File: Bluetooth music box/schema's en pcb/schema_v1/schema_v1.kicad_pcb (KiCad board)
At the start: 4 copper layers, 141 x 87.6 mm, 151 parts, among them J1 Pickit aansluiting, J2 USB_B_Micro, SW1 SW_Push, SW3 SW_Push, SW4 SW_Push, SW5 SW_Push, SW6 SW_Push, SW7 SW_Push, SW9 Switch, U1 LTC2063, U10 SN74LVC1T45DBV, U11 tpa3140, U12 LTC4001, U14 TPS563200, U2 pic18f27k40, U5 FT232RL, U6 LM1117-3.3, U8 OVC3860_EDR, U9 Spi_header

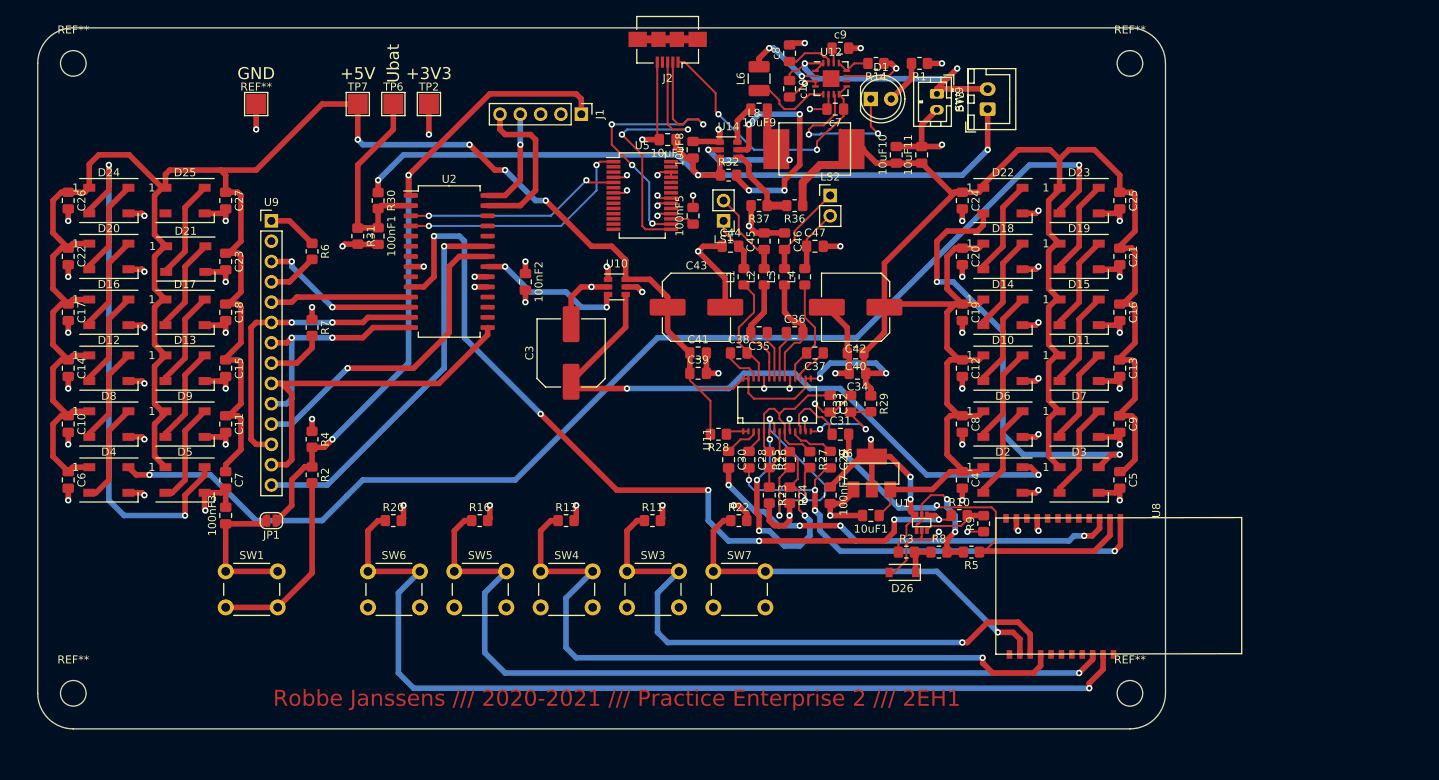
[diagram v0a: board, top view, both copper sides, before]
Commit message: Nieuwe start
Nieuw schema (andere µC, BT-module, dc/dc, verschillversterkers)
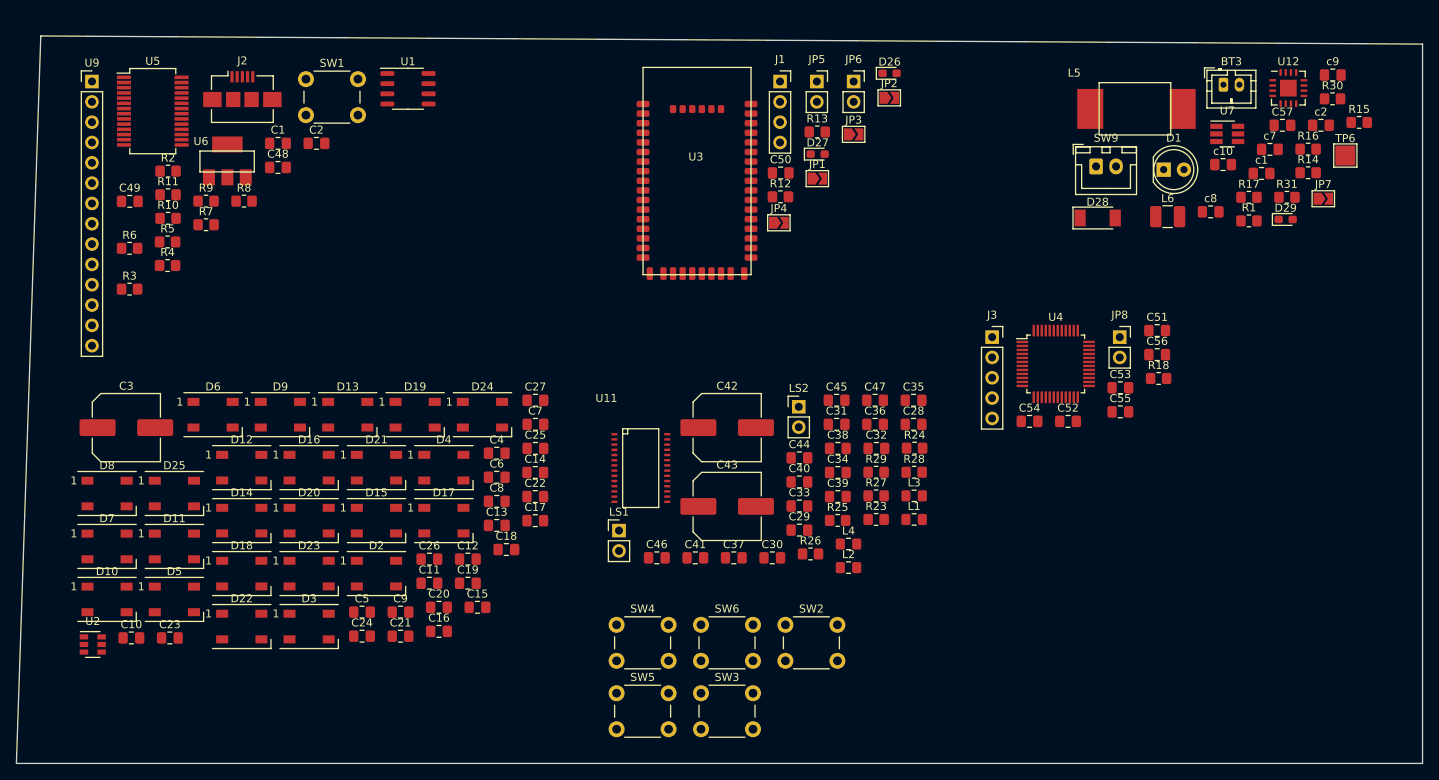
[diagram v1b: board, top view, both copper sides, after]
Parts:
- removed 100nF1, 100nF2, 100nF3, 100nF5, 100nF7, 10uF1, 10uF7, 10uF8: C, Capacitor_SMD:C_0805_2012Metric_Pad1.18x1.45mm_HandSolder
- removed 10uF10, 10uF11: 22µF, Capacitor_SMD:C_0805_2012Metric_Pad1.18x1.45mm_HandSolder
- removed 10uF9: 0.1µF, Capacitor_SMD:C_0805_2012Metric_Pad1.18x1.45mm_HandSolder
- removed L8: 2.2uH, Robbe_modules:L_tps563200
- removed R20, R22, R32, R37: 10k, Resistor_SMD:R_0805_2012Metric_Pad1.20x1.40mm_HandSolder
- removed R36: 56k, Resistor_SMD:R_0805_2012Metric_Pad1.20x1.40mm_HandSolder
- removed REF**: TestPoint_GND, TestPoint:TestPoint_Pad_2.5x2.5mm
- removed REF** (x4): MountingHole_3.2mm_M3, MountingHole:MountingHole_3.2mm_M3
- removed SW7: SW_Push, Button_Switch_THT:SW_PUSH_6mm_H7.3mm
- removed TP2, TP7: TestPoint, TestPoint:TestPoint_Pad_2.5x2.5mm
- removed U10: SN74LVC1T45DBV, Package_TO_SOT_SMD:SOT-23-6
- removed U14: TPS563200, Package_TO_SOT_SMD:SOT-23-6
- removed U8: OVC3860_EDR, Robbe_modules:OVC3860_EDR
- added C1: 100nF, Capacitor_SMD:C_0805_2012Metric_Pad1.18x1.45mm_HandSolder, F.Cu at (106.9, 62.7)
- added C2: 10uF, Capacitor_SMD:C_0805_2012Metric_Pad1.18x1.45mm_HandSolder, F.Cu at (111.7, 62.7)
- added C48: 100nF, Capacitor_SMD:C_0805_2012Metric_Pad1.18x1.45mm_HandSolder, F.Cu at (106.9, 65.7)
- added C49: 100nF, Capacitor_SMD:C_0805_2012Metric_Pad1.18x1.45mm_HandSolder, F.Cu at (88.3, 70.0)
- added C50: 10uF, Capacitor_SMD:C_0805_2012Metric_Pad1.18x1.45mm_HandSolder, F.Cu at (169.7, 66.4)
- added C51: 100nF, Capacitor_SMD:C_0805_2012Metric_Pad1.18x1.45mm_HandSolder, F.Cu at (216.8, 86.1)
- added C52: 100nF, Capacitor_SMD:C_0805_2012Metric_Pad1.18x1.45mm_HandSolder, F.Cu at (205.6, 97.5)
- added C53: 100nF, Capacitor_SMD:C_0805_2012Metric_Pad1.18x1.45mm_HandSolder, F.Cu at (212.2, 93.3)
- added C54: 100nF, Capacitor_SMD:C_0805_2012Metric_Pad1.18x1.45mm_HandSolder, F.Cu at (200.8, 97.5)
- added C55: 100nF, Capacitor_SMD:C_0805_2012Metric_Pad1.18x1.45mm_HandSolder, F.Cu at (212.2, 96.3)
- added C56: 10nF, Capacitor_SMD:C_0805_2012Metric_Pad1.18x1.45mm_HandSolder, F.Cu at (216.8, 89.1)
- added C57: 100nF, Capacitor_SMD:C_0805_2012Metric_Pad1.18x1.45mm_HandSolder, F.Cu at (232.4, 60.4)
- added D27: RED, LED_SMD:LED_0603_1608Metric_Pad1.05x0.95mm_HandSolder, F.Cu at (174.3, 64.0)
- added D28: D_Schottky, Diode_SMD:D_SOD-128, F.Cu at (209.3, 72.0)
- added D29: RED, LED_SMD:LED_0603_1608Metric_Pad1.05x0.95mm_HandSolder, F.Cu at (232.8, 72.2)
- added J3: Conn_01x05_Male, Connector_PinSocket_2.54mm:PinSocket_1x05_P2.54mm_Vertical, F.Cu at (196.1, 86.9)
- added JP2: SolderJumper, Jumper:SolderJumper-2_P1.3mm_Open_TrianglePad1.0x1.5mm, F.Cu at (183.3, 57.0)
- added JP3: SolderJumper, Jumper:SolderJumper-2_P1.3mm_Open_TrianglePad1.0x1.5mm, F.Cu at (178.8, 61.6)
- added JP4: SolderJumper, Jumper:SolderJumper-2_P1.3mm_Open_TrianglePad1.0x1.5mm, F.Cu at (169.5, 72.6)
- added JP5: Jumper, Connector_PinSocket_2.54mm:PinSocket_1x02_P2.54mm_Vertical, F.Cu at (174.2, 55.0)
- added JP6: Jumper, Connector_PinSocket_2.54mm:PinSocket_1x02_P2.54mm_Vertical, F.Cu at (178.8, 55.0)
- added JP7: SolderJumper, Jumper:SolderJumper-2_P1.3mm_Open_TrianglePad1.0x1.5mm, F.Cu at (237.5, 69.6)
- added JP8: Jumper, Connector_PinSocket_2.54mm:PinSocket_1x02_P2.54mm_Vertical, F.Cu at (212.1, 86.9)
- added L5: 2.2uH, Robbe_modules:L_tps563200, F.Cu at (206.4, 53.4)
- added R12: 100, Resistor_SMD:R_0805_2012Metric_Pad1.20x1.40mm_HandSolder, F.Cu at (169.7, 69.4)
- added R15: 562K, Resistor_SMD:R_0805_2012Metric_Pad1.20x1.40mm_HandSolder, F.Cu at (242.0, 60.1)
- added R17: 100, Resistor_SMD:R_0805_2012Metric_Pad1.20x1.40mm_HandSolder, F.Cu at (228.2, 69.4)
- added R18: 10K, Resistor_SMD:R_0805_2012Metric_Pad1.20x1.40mm_HandSolder, F.Cu at (216.9, 92.1)
- added SW2: SW_Push, Button_Switch_THT:SW_PUSH_6mm_H7.3mm, F.Cu at (170.3, 122.9)
- added U3: RN52, Robbe_modules:RN52, F.Cu at (152.5, 79.1)
- added U4: STM32L443CCTx, Package_QFP:LQFP-48_7x7mm_P0.5mm, F.Cu at (204.1, 90.3)
- added U7: TLV61048, Package_TO_SOT_SMD:SOT-23-6_Handsoldering, F.Cu at (225.5, 61.5)
- added c1: 1uF, Capacitor_SMD:C_0805_2012Metric_Pad1.18x1.45mm_HandSolder, F.Cu at (229.8, 66.5)
- added c2: 10µF, Capacitor_SMD:C_0805_2012Metric_Pad1.18x1.45mm_HandSolder, F.Cu at (237.2, 60.4)
- D26: value D_Zener -> BLUE; footprint Diode_SMD:D_SOD-123 -> LED_SMD:LED_0603_1608Metric_Pad1.05x0.95mm_HandSolder
- J1: value Pickit aansluiting -> Conn_01x04; footprint Connector_PinHeader_2.54mm:PinHeader_1x05_P2.54mm_Vertical -> Connector_PinSocket_2.54mm:PinSocket_1x04_P2.54mm_Vertical
- JP1: footprint Jumper:SolderJumper-2_P1.3mm_Open_RoundedPad1.0x1.5mm -> Jumper:SolderJumper-2_P1.3mm_Open_TrianglePad1.0x1.5mm
- R10, R11, R4: value 10k -> 220K
- R13: value 10k -> 100
- R16: value 10k -> 107K
- R2: value 100 -> 100K
- R3: value 10k -> 100K
- R5: value 100k -> 220K
- R8, R9: value 100k -> 100K
- U1: value LTC2063 -> TL072; footprint Robbe_modules:LTC2063 -> Package_SO:SO-8_3.9x4.9mm_P1.27mm
- U2: value pic18f27k40 -> SN74LVC1T45DBV; footprint Package_SO:SOIC-28W_7.5x18.7mm_P1.27mm -> Package_TO_SOT_SMD:SOT-23-6
- moved D7 122.5 mm to (85.5, 113.1)
- moved R30 120.0 mm to (238.7, 57.1), turned to 0 degrees
- moved TP6 119.2 mm to (240.3, 64.2)
- moved R31 116.2 mm to (233.0, 69.4), turned to 0 degrees
- moved D10 115.7 mm to (85.5, 119.7)
- moved D11 115.3 mm to (93.9, 113.1)
- moved R16 113.5 mm to (235.6, 63.4)
- moved D22 109.0 mm to (102.3, 123.1)
- moved R5 107.7 mm to (93.1, 75.0), turned to 0 degrees
- moved D23 107.0 mm to (110.8, 116.5)
- moved R10 105.6 mm to (93.1, 72.1)
- moved R9 105.2 mm to (97.9, 69.9), turned to 0 degrees
- moved D18 103.1 mm to (102.3, 116.5)
- moved R3 102.5 mm to (88.3, 80.9)
- moved C21 101.7 mm to (122.2, 124.3), turned to 0 degrees
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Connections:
- C28 pad 2: /Class d amplifier/Agnd -> /L-
- C29 pad 2: /Class d amplifier/Agnd -> /R-
- C3 pad 1: DataLeds -> +5V
- C30 pad 2: /Class d amplifier/Aleft -> /L+
- C31 pad 2: VoL_Measure -> /R+
- D2 pad 4: DataLeds -> /LEDS/FirstLED
- D26 pad 2: GND -> +3V3
- J1 pad 1: Reset -> Net-(J1-Pad1)
- J1 pad 2: +3V3 -> Net-(J1-Pad2)
- J1 pad 3: GND -> Net-(J1-Pad3)
- J1 pad 4: PGD -> Net-(J1-Pad4)
- JP1 pad 1: Reset -> RTS_BT
- JP1 pad 2: Net-(100nF3-Pad1) -> Net-(J1-Pad1)
- R10 pad 1: Vol_spkr -> GND
- R11 pad 1: vol+ -> /R_SE
- R11 pad 2: GND -> Net-(R11-Pad2)
- R13 pad 1: vol- -> Net-(R13-Pad1)
- R13 pad 2: GND -> Net-(D27-Pad1)
- R16 pad 1: next -> Net-(R15-Pad2)
- R2 pad 1: Reset -> Net-(R2-Pad1)
- R2 pad 2: Net-(R2-Pad2) -> /L+
- R3 pad 1: +3V3 -> Net-(R3-Pad1)
- R3 pad 2: Net-(D26-Pad1) -> /L-
- R4 pad 1: +3V3 -> GND
- R4 pad 2: Reset -> Net-(R3-Pad1)
- R5 pad 1: VoL_Measure -> /L_SE
- R5 pad 2: Net-(R5-Pad2) -> Net-(R2-Pad1)
- R6 pad 2: LCS_rst -> LCD_rst
- R8 pad 1: Net-(D26-Pad1) -> Net-(R11-Pad2)
- R8 pad 2: Net-(R5-Pad2) -> /R+
- R9 pad 1: GND -> Net-(R10-Pad2)
- R9 pad 2: Net-(R10-Pad2) -> /R-
- SW1 pad 1: Net-(100nF3-Pad1) -> GND
- SW1 pad 2: Net-(R2-Pad2) -> Reset
- SW3 pad 1: vol+ -> GND
- SW3 pad 2: +3V3 -> vol-
- SW4 pad 1: vol- -> GND
- SW4 pad 2: +3V3 -> next
- SW5 pad 1: next -> GND
- SW5 pad 2: +3V3 -> prev
- SW6 pad 1: prev -> GND
- SW6 pad 2: +3V3 -> pp
- U1 pad 1: Net-(R5-Pad2) -> /L_SE
- U1 pad 2: GND -> Net-(R3-Pad1)
- U1 pad 3: Net-(R10-Pad2) -> Net-(R2-Pad1)
- U1 pad 4: Vol_spkr -> GND
- U1 pad 5: Net-(R5-Pad2) -> Net-(R11-Pad2)
- U1 pad 6: +3V3 -> Net-(R10-Pad2)
- U2 pad 1: Reset -> +3V3
- U2 pad 2: BAT_ADC -> GND
- U2 pad 3: TX -> /LEDS/D_LEDS
- U2 pad 4: RX -> /LEDS/FirstLED
- U2 pad 5: RA3 -> +3V3
- U2 pad 6: Net-(U2-Pad6) -> +5V
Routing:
- net +5V: track 555.4 -> 0.00 mm, vias 6 -> 0
- net GND: track 269.1 -> 0.00 mm, vias 75 -> 0
- net Net-(D23-Pad2): track 147.1 -> 0.00 mm, vias 2 -> 0
- net prev: track 120.2 -> 0.00 mm, vias 1 -> 0
- net next: track 103.9 -> 0.00 mm, vias 1 -> 0
- net Vol_spkr: track 102.0 -> 0.00 mm, vias 6 -> 0
- net Vbat: track 98.2 -> 0.00 mm, vias 3 -> 0
- net vol-: track 88.0 -> 0.00 mm, vias 1 -> 0
- net Reset: track 82.1 -> 0.00 mm, vias 2 -> 0
- net DataLeds: track 80.9 -> 0.00 mm, vias 2 -> 0
- net vol+: track 74.3 -> 0.00 mm, vias 1 -> 0
- net Net-(D24-Pad2): track 66.3 -> 0.00 mm, vias 2 -> 0
- net /Class d amplifier/Agnd: track 62.1 -> 0.00 mm, vias 4 -> 0
- net +3V3: track 57.0 -> 0.00 mm, vias 14 -> 0
- net Net-(D22-Pad2): track 55.8 -> 0.00 mm, vias 2 -> 0
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- removed copper zone on In1.Cu, net +3V3
- removed copper zone on In2.Cu, net GND
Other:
- board size 141 x 87.6 mm -> 175.8 x 90.9 mm
- board text removed: "+3V3"
- board text removed: "+5V"
- board text removed: "GND"
- board text removed: "Robbe Janssens /// 2020-2021 /// Practice Enterprise 2 /// 2EH1"
- board text removed: "Ubat"
